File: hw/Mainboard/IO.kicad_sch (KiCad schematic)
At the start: 10 parts, among them U7 W65C21N, U8 W65C21N, U9 W65C22N

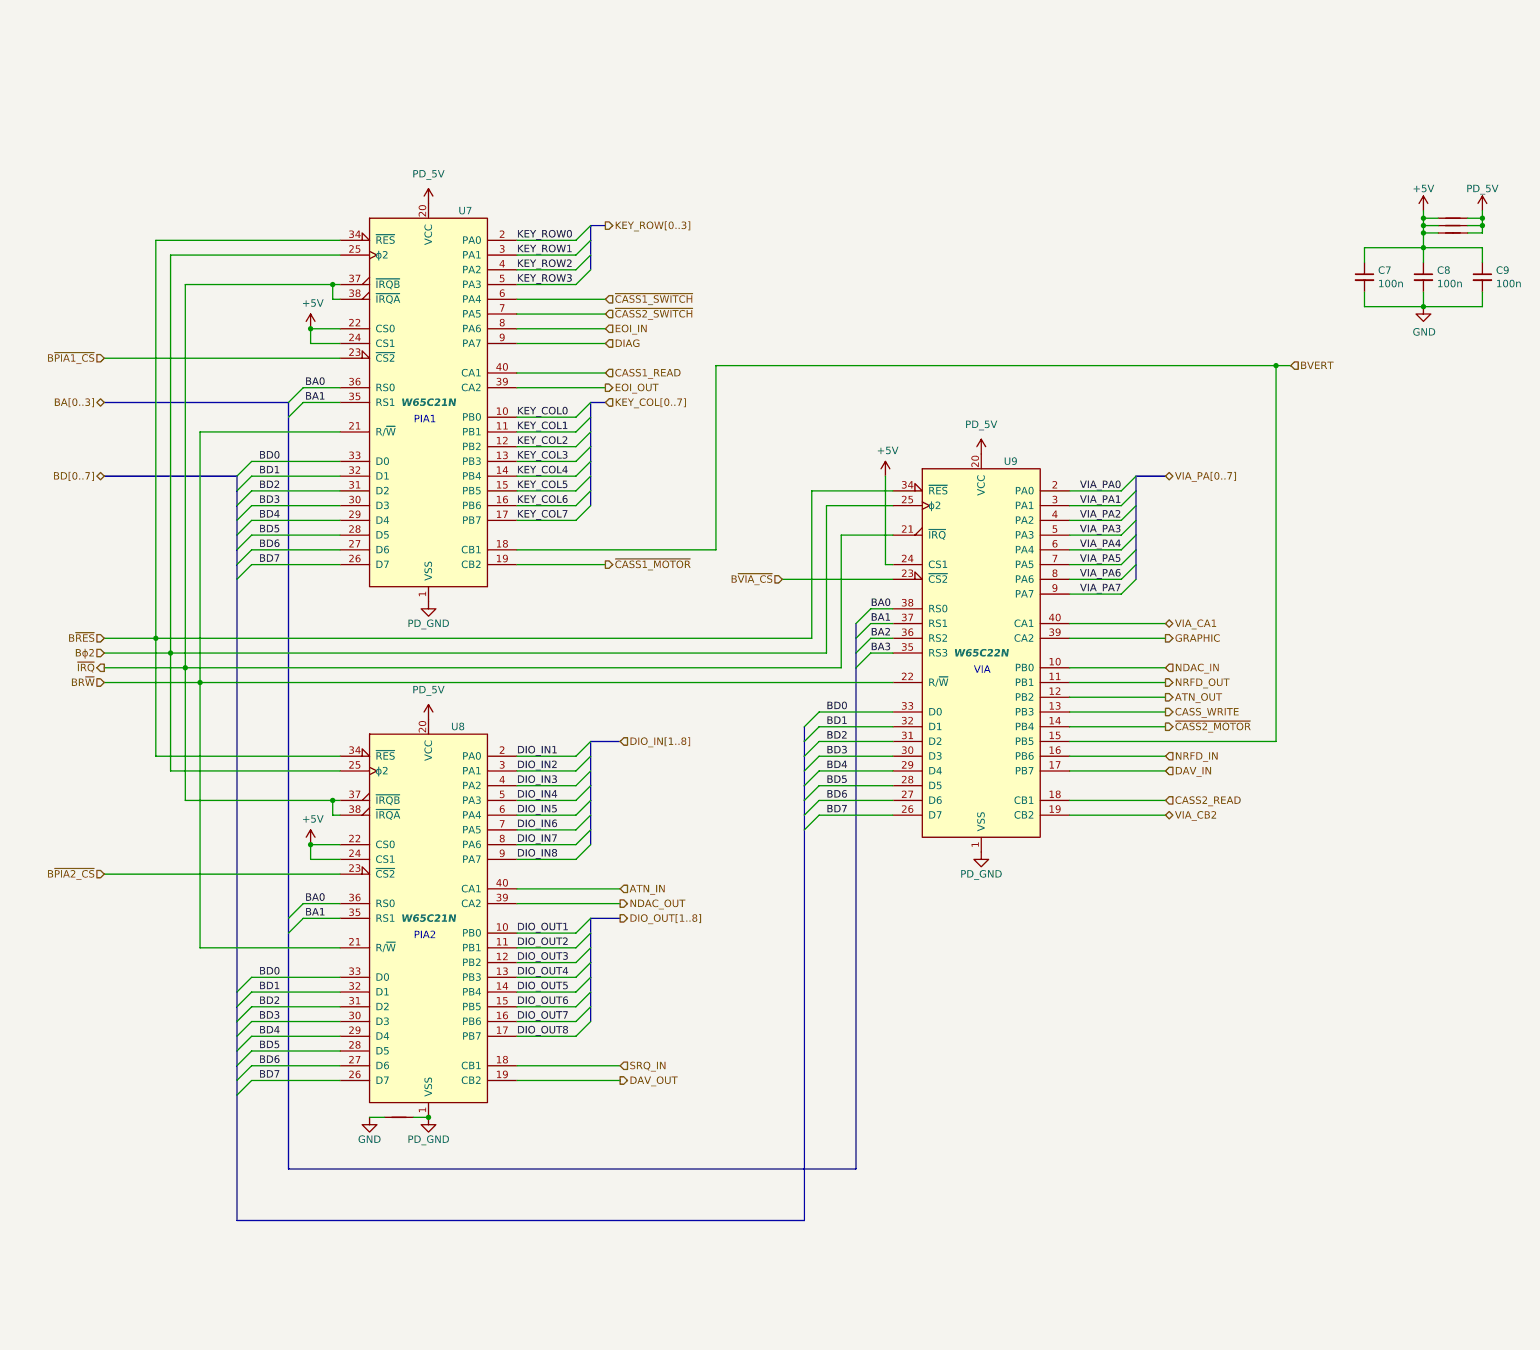
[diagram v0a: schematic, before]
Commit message: hw: wip
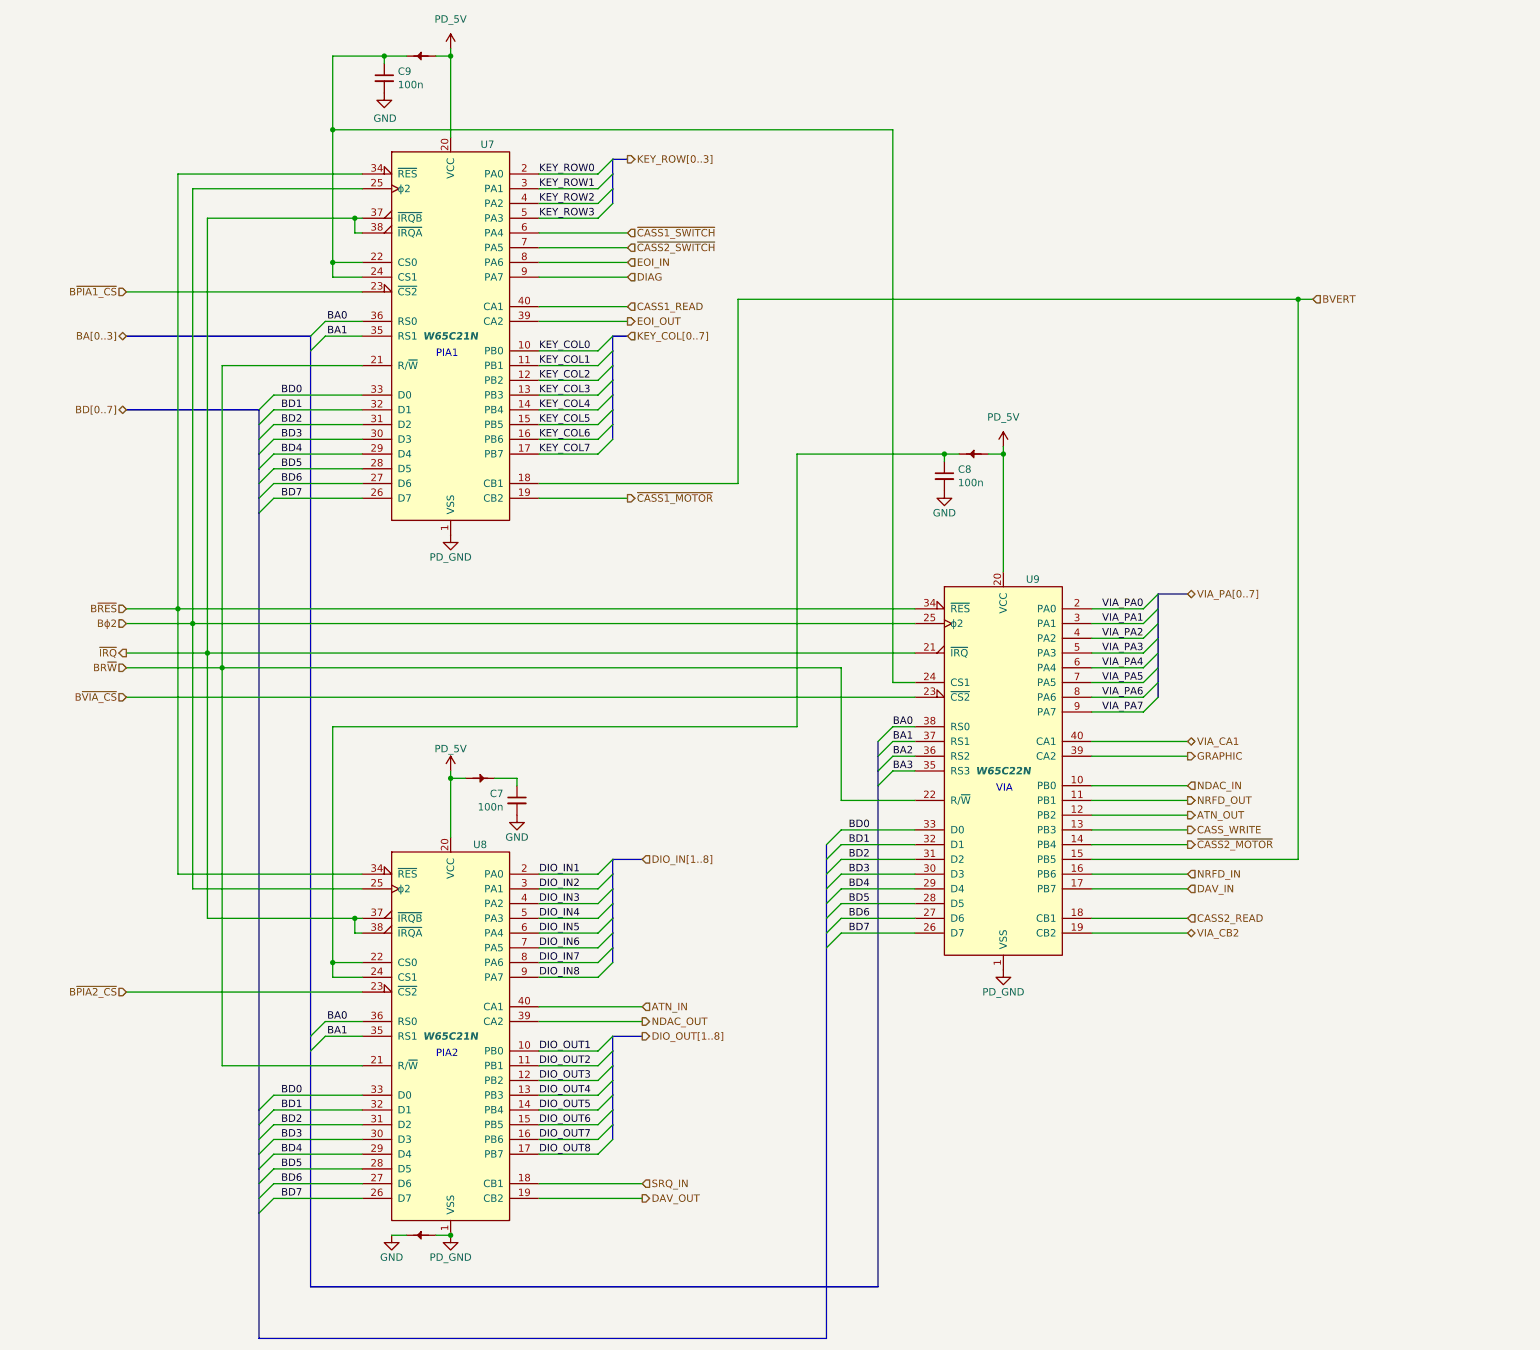
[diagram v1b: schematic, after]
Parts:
- NT10, NT13, NT14, NT15: symbol Device:NetTie_2 -> PET:PowerTie_2
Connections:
- removed net +5V: C7.1, C8.1, C9.1, NT10.2, NT13.2, NT14.2, U7.22 (CS0), U7.24 (CS1), U8.22 (CS0), U8.24 (CS1), U9.24 (CS1)
- new net: C8.1, NT13.2, U8.22 (CS0), U8.24 (CS1)
- new net: C9.1, NT10.2, U7.22 (CS0), U7.24 (CS1), U9.24 (CS1)
- new net: C7.1, NT14.2
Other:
- moved on the sheet: C7, C8, C9, U7, U8, U9
